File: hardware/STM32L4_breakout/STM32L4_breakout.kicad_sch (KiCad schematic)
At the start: 64 parts, among them J1 12V IN, J10 GPIO, J11 SPI1, J12 USART1, J13 USART3, J14 UART4, J15 3.3V, J16 5V, J17 12V, J2 SWD, J3 Conn_01x08, J4 Conn_01x06, J5 Conn_01x10, J6 Conn_01x08, J7 I2C1, J8 I2C2, J9 I2C3, SW1 SW_SPDT, U1 LD1117S50TR_SOT223, U2 LD3985M33R_SOT23, U3 LD1117S33TR_SOT223, U4 STM32L476RGTx, X1 NX3215SA-32.768K

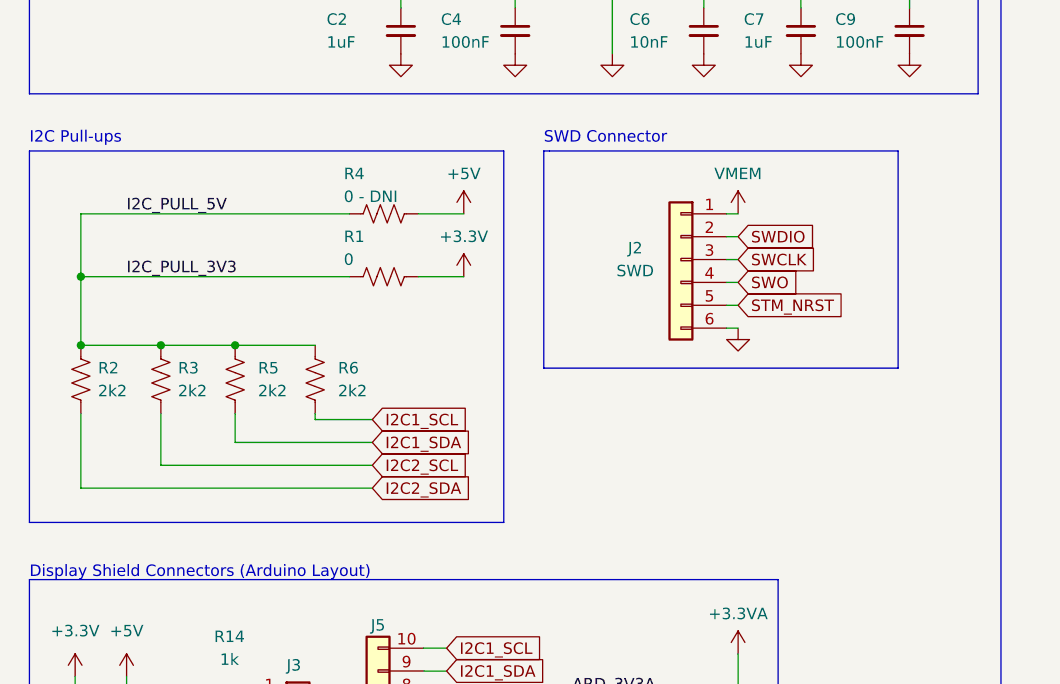
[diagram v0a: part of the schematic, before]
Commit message: breakout board pcb layout WIP - ready for outline
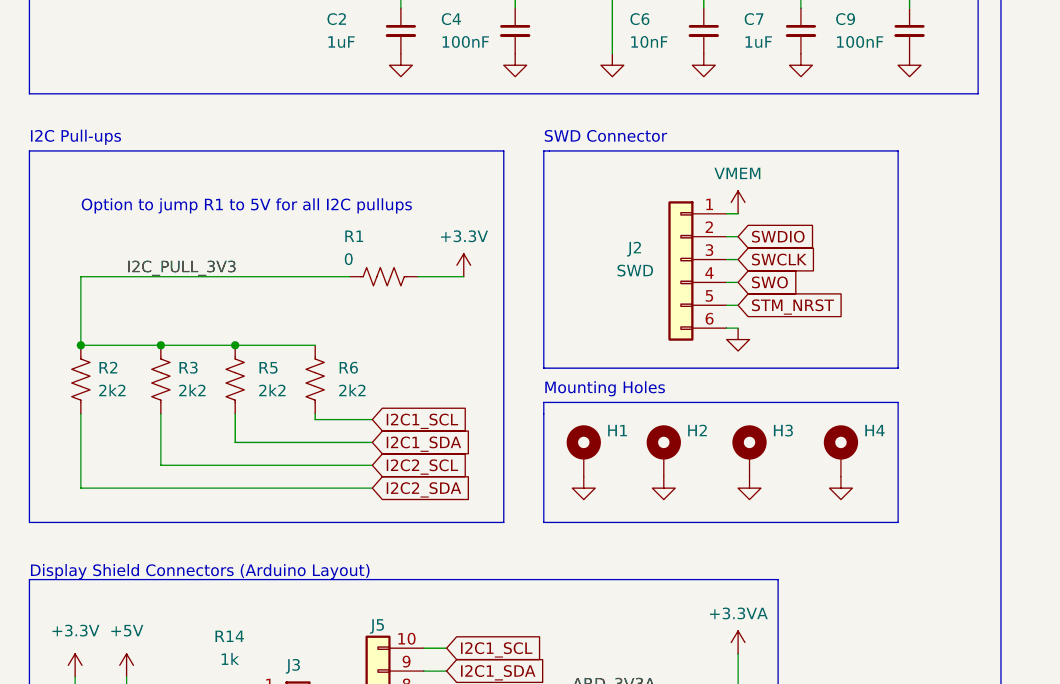
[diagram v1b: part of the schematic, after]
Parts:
- removed R4: 0 - DNI, Resistor_SMD:R_0603_1608Metric, symbol Device:R_US
- added H1, H2, H3, H4: MountingHole_Pad, MountingHole:MountingHole_3.2mm_M3_DIN965_Pad_TopOnly, symbol Mechanical:MountingHole_Pad
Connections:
- net GND: now also H1.1, H2.1, H3.1, H4.1
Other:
- note added: "Mounting Holes"
- note added: "Option to jump R1 to 5V for all I2C pullups"
